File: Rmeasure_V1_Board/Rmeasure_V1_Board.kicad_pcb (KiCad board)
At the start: 2 copper layers, 58 x 28.5 mm, 49 parts, among them J1 USB_C_Receptacle_USB2.0, J2 CON_debug, J3 Conn_ARM_JTAG_SWD_10, J4 CON_CAN, J5 CON_CAN, U1 STM32F302C6Tx, U2 NCP1117-3.3_SOT223, U3 SN65HVD232, Y1 8MHz

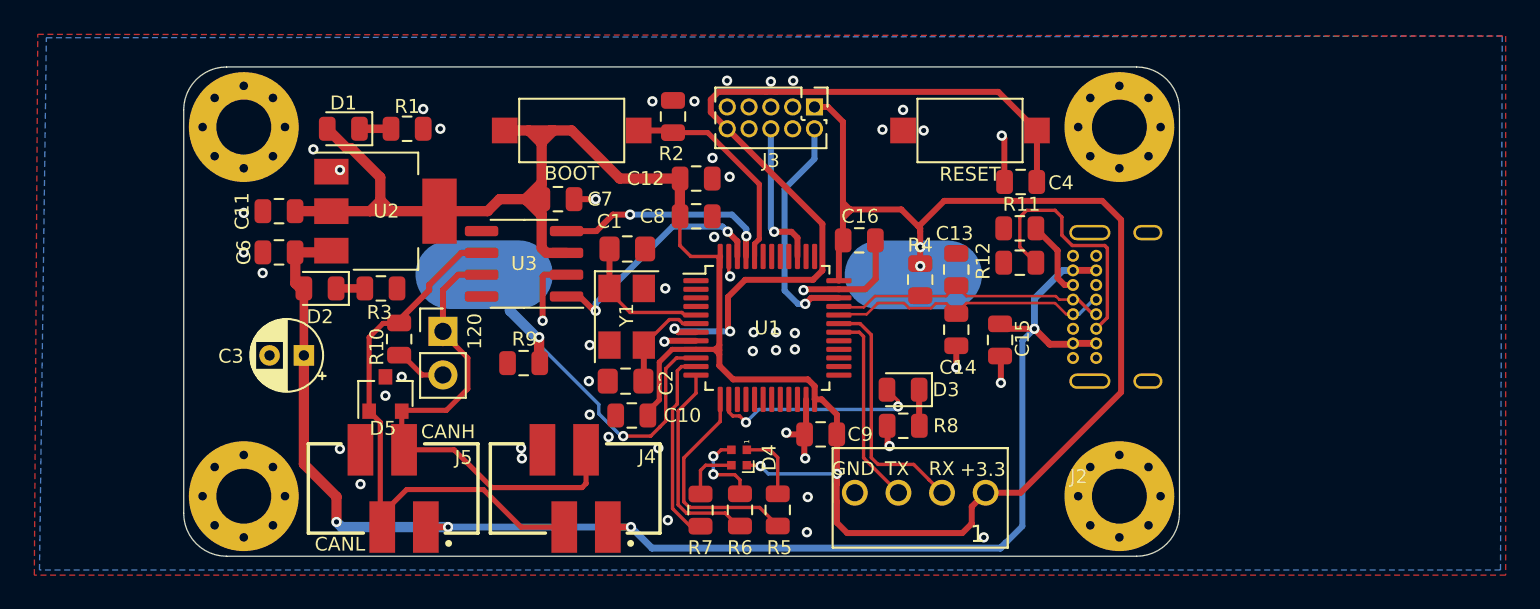
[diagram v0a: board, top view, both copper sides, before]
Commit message: lots of stuf
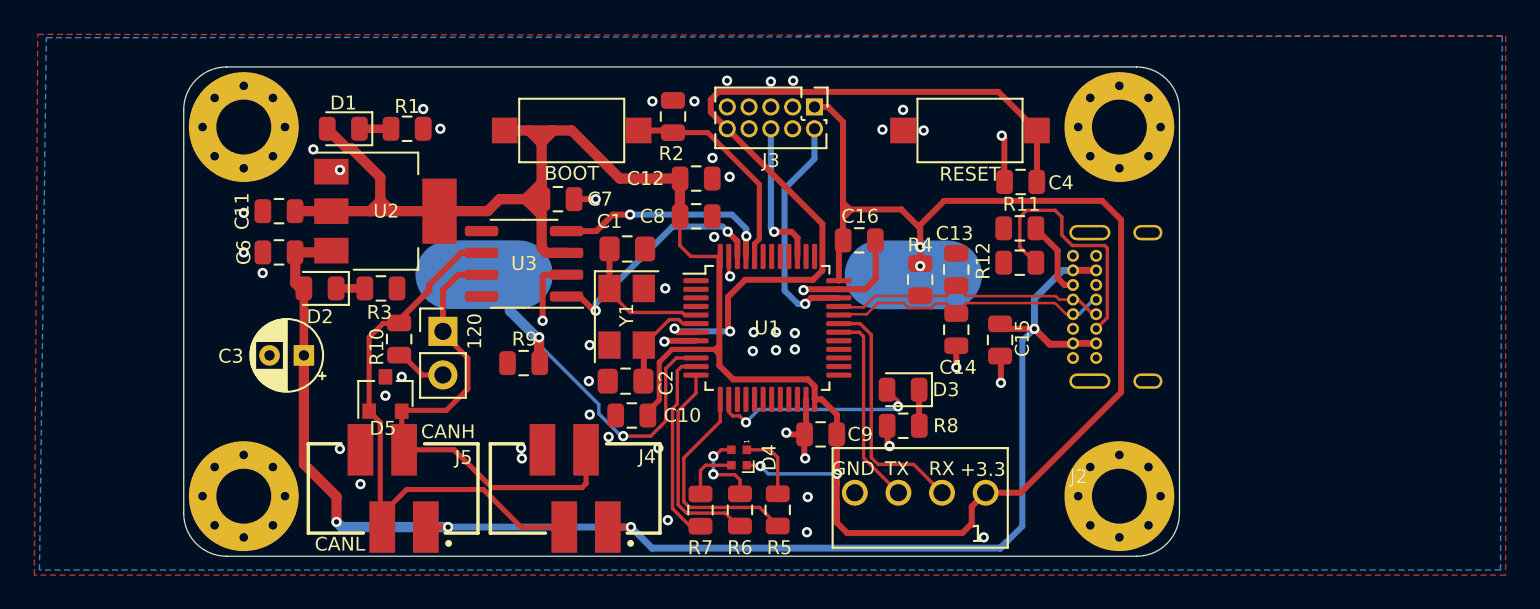
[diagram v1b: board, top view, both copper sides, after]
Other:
- net class Default removed
